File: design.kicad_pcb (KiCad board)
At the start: 2 copper layers, 25 x 22.9 mm, 14 parts, among them J1 Conn_01x02, J2 Conn_01x02, J3 Conn_01x03, J4 Conn_01x03, U1 TPS61099YFFT

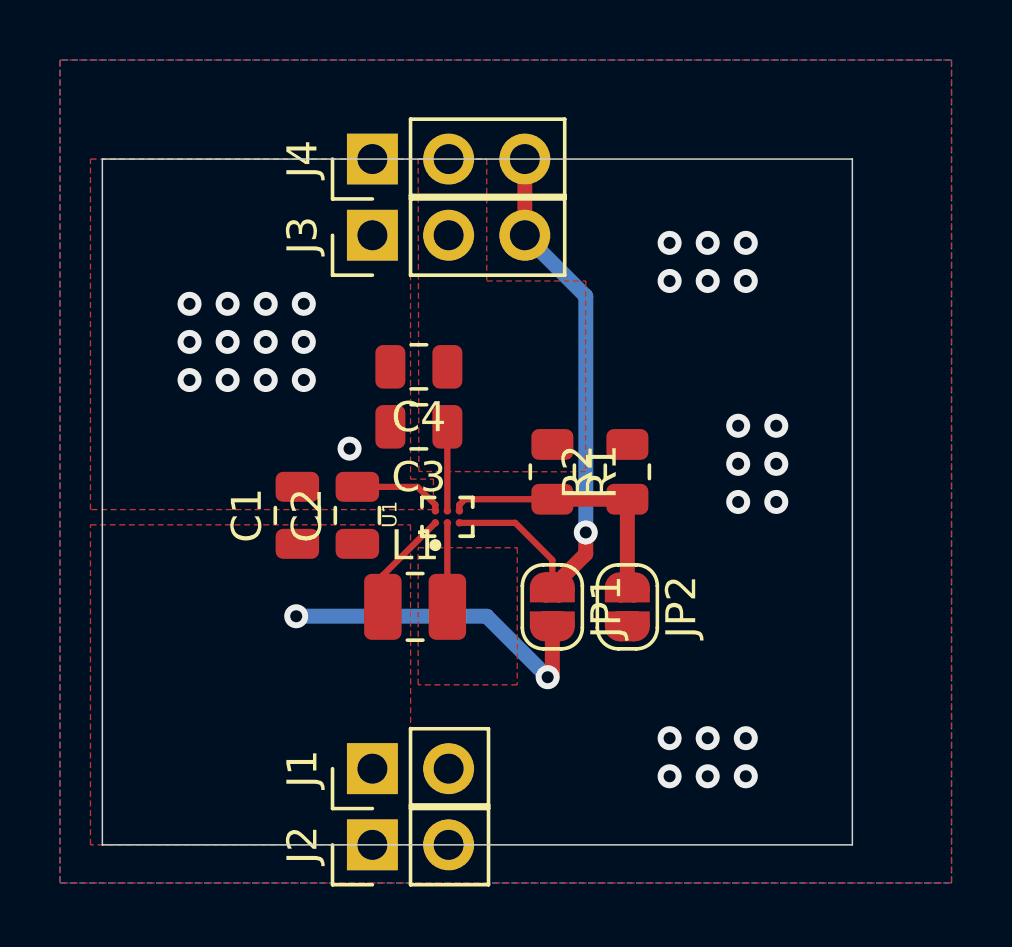
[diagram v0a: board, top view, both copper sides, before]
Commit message: PCB Move Silkscreen
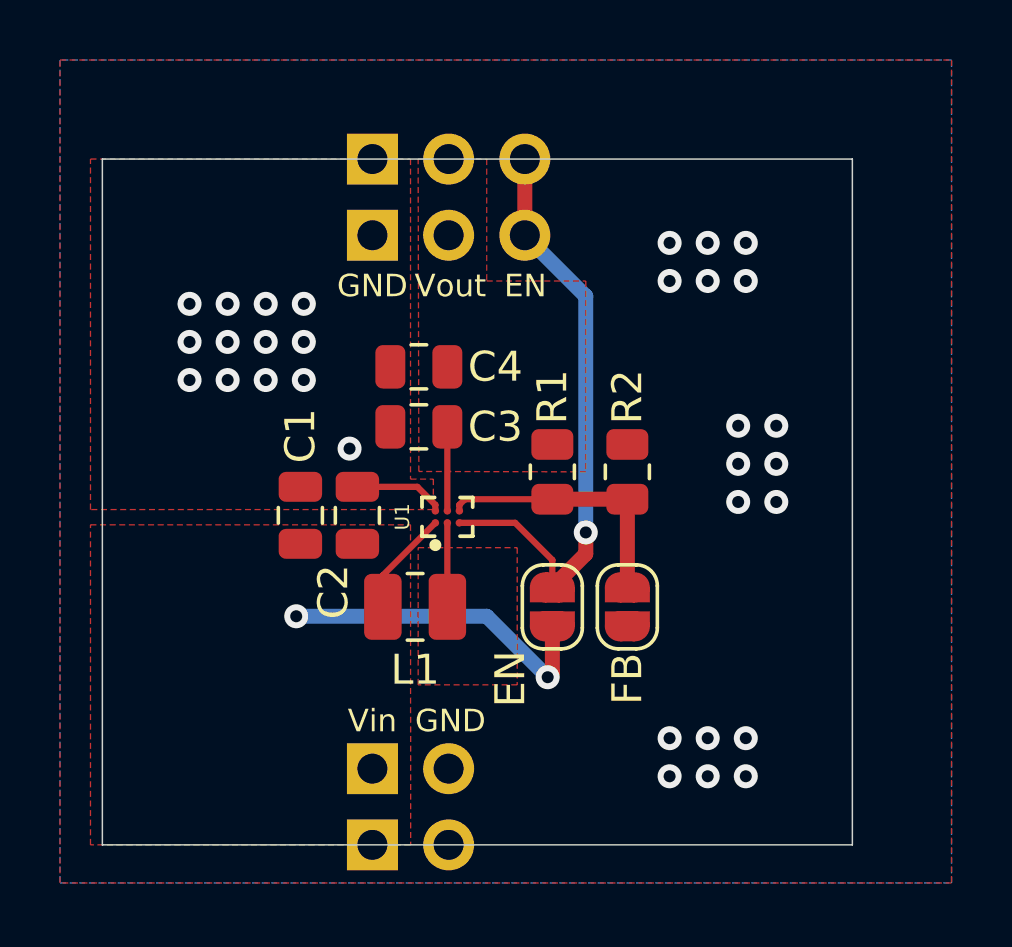
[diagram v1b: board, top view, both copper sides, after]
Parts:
- moved C1 0.10 mm to (140.6, 96.0)
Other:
- board text added: "EN"
- board text added: "GND"
- board text added: "Vin"
- board text added: "Vout"
